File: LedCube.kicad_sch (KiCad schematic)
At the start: 0 parts

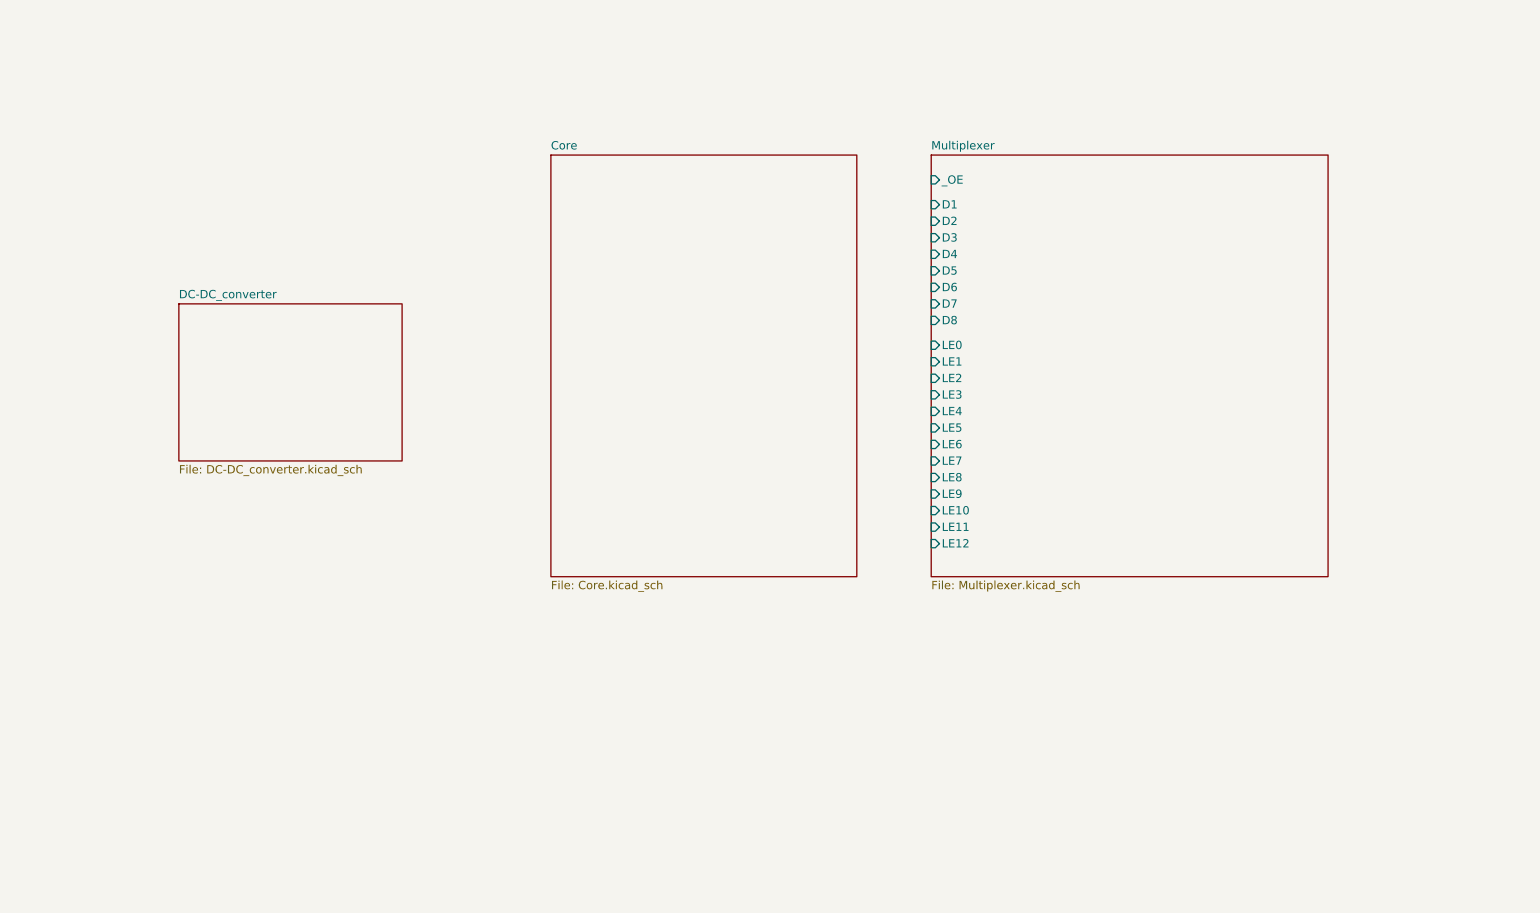
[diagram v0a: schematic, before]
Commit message: Schematic + PCB
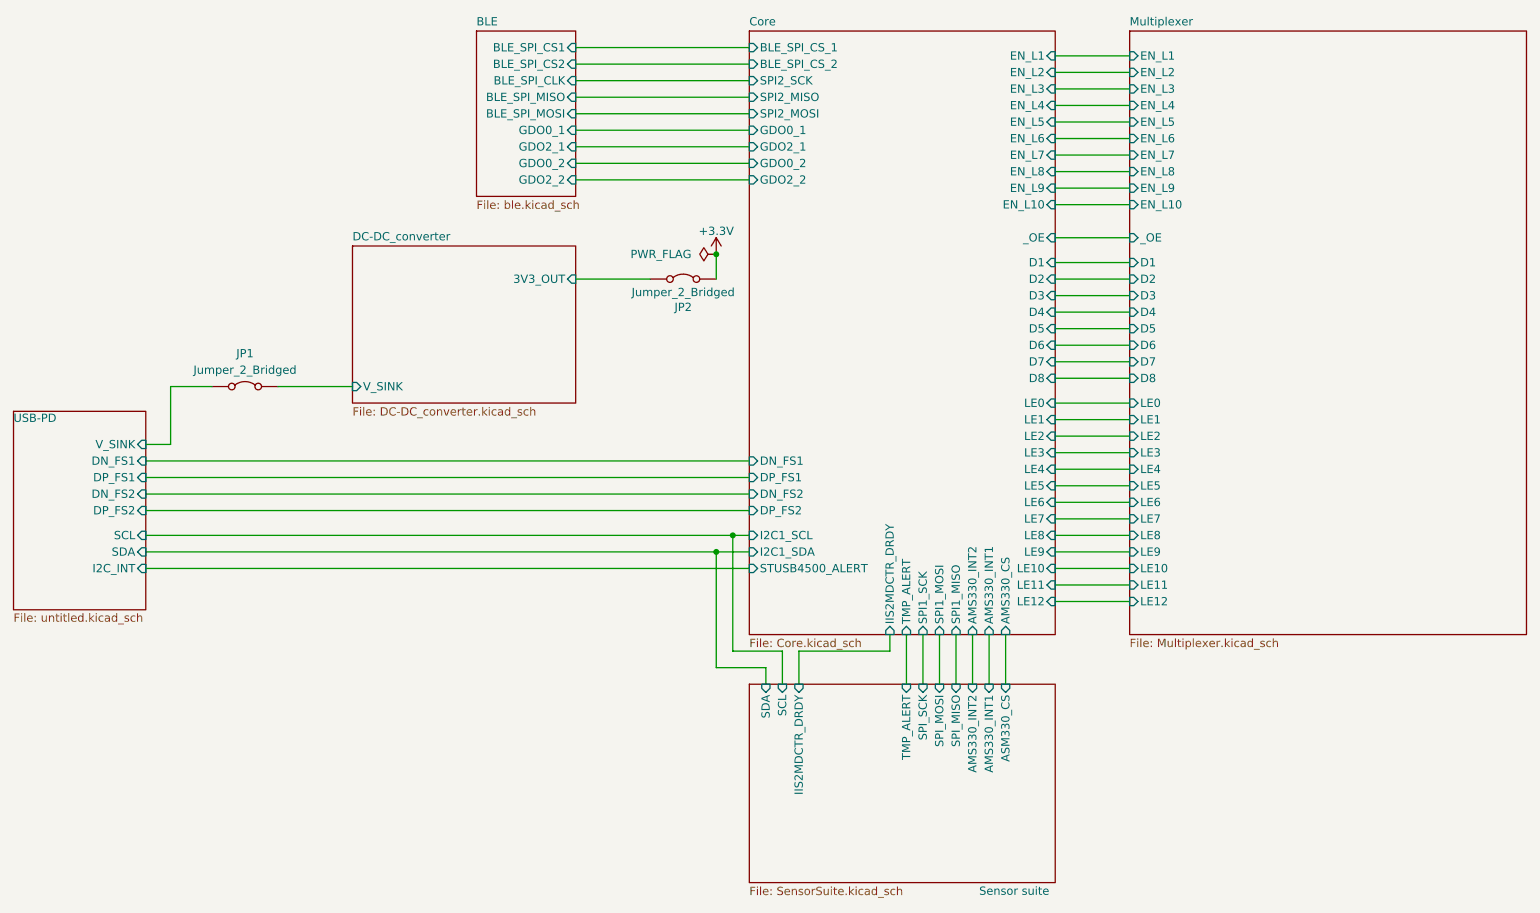
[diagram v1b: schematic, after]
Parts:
- added JP1, JP2: Jumper_2_Bridged, Resistor_SMD:R_0805_2012Metric, symbol Jumper:Jumper_2_Bridged
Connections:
- new net +3.3V: JP2.2 (B)
- new net DC-DC_converter/3V3_OUT: JP2.1 (A)
- new net DC-DC_converter/V_SINK: JP1.2 (B)
- new net USB-PD/V_SINK: JP1.1 (A)
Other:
- added sheet BLE (ble.kicad_sch)
- added sheet Sensor suite (SensorSuite.kicad_sch)
- added sheet USB-PD (untitled.kicad_sch)
- sheet Core ports: added AMS330_CS, AMS330_INT1, AMS330_INT2, BLE_SPI_CS_1, BLE_SPI_CS_2, D1, D2, D3, D4, D5, D6, D7, D8, DN_FS1, DN_FS2, DP_FS1, DP_FS2, EN_L1, EN_L10, EN_L2, EN_L3, EN_L4, EN_L5, EN_L6, EN_L7, EN_L8, EN_L9, GDO0_1, GDO0_2, GDO2_1, GDO2_2, I2C1_SCL, I2C1_SDA, IIS2MDCTR_DRDY, LE0, LE1, LE10, LE11, LE12, LE2, LE3, LE4, LE5, LE6, LE7, LE8, LE9, SPI1_MISO, SPI1_MOSI, SPI1_SCK, SPI2_MISO, SPI2_MOSI, SPI2_SCK, STUSB4500_ALERT, TMP_ALERT, _OE; removed none
- sheet DC-DC_converter ports: added 3V3_OUT, V_SINK; removed none
- sheet Multiplexer ports: added EN_L1, EN_L10, EN_L2, EN_L3, EN_L4, EN_L5, EN_L6, EN_L7, EN_L8, EN_L9; removed none
